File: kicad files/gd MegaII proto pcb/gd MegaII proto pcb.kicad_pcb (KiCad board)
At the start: 4 copper layers, 60 parts, among them J1 ABDIR, J10 Data, J11 PWR, J12 CLKS, J2 ABEN, J3 FLIP, J4 DBDIR, J5 DBEN, J6 VGC Extra 1, J7 Bald-Ext-1, J8 VGC Extra 2, J9 Address, U1 Apple_MEGA_II, U2 DRAM64KX4, U3 74HCT245, U4 DRAM64KX4, U5 74HCT245, U6 74HCT86, U7 DRAM64KX4, U8 74HCT245, U9 DRAM64KX4

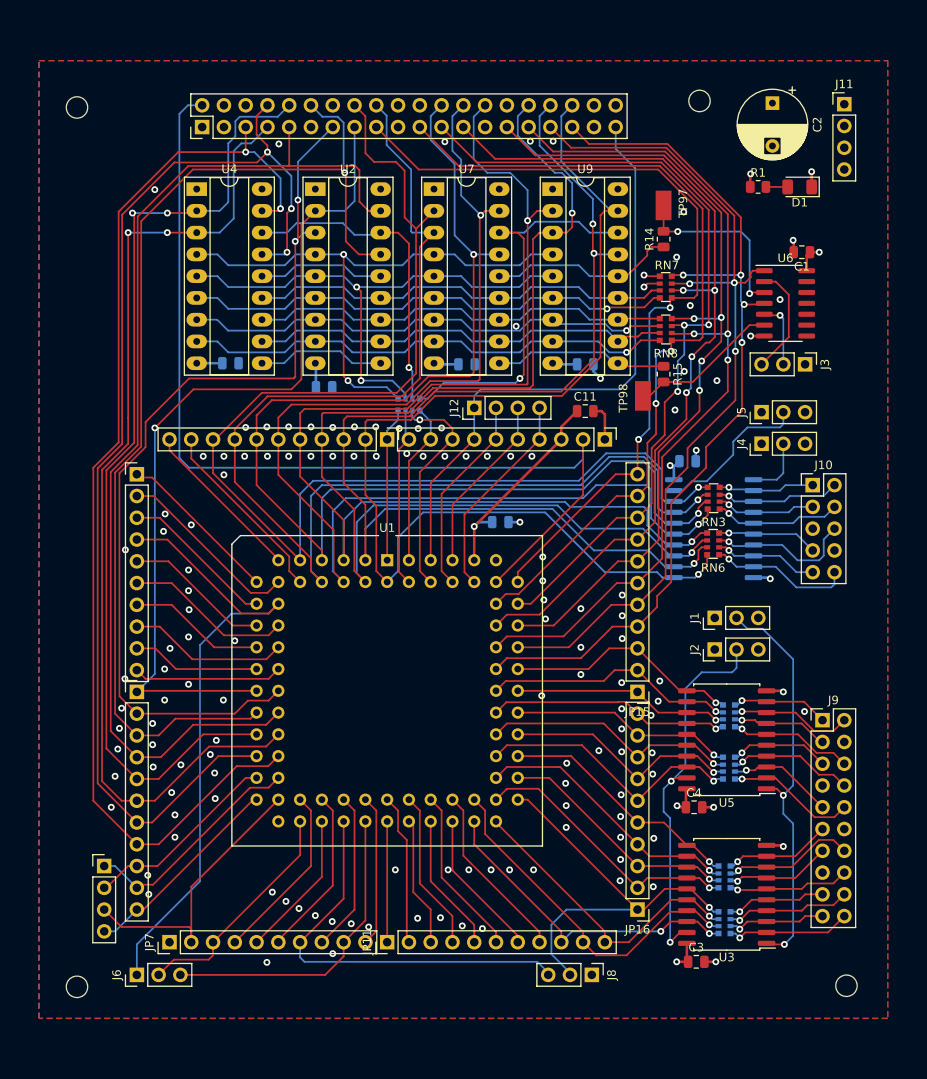
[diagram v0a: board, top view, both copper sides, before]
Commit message: all three boards final, prepping for gerbers
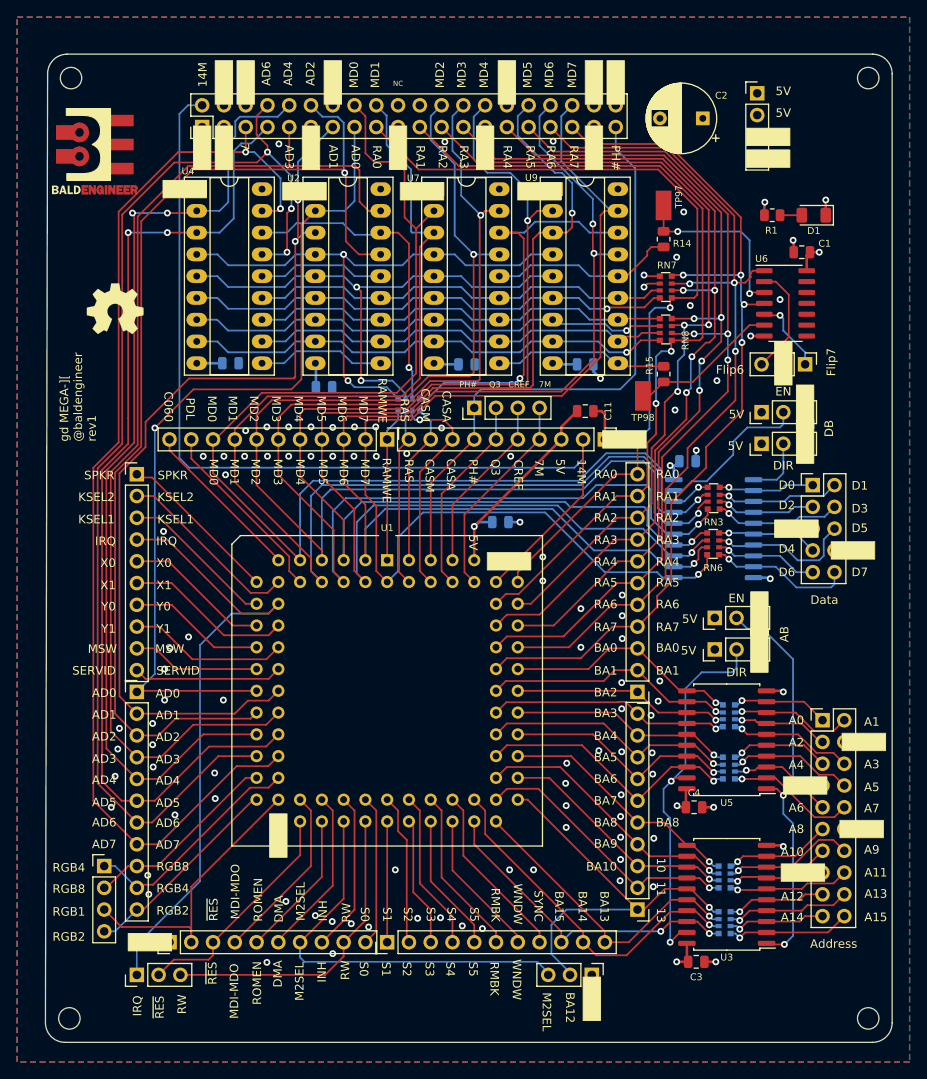
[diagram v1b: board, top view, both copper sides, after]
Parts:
- added REF**: OSHW-Symbol_6.7x6mm_SilkScreen, Symbol:OSHW-Symbol_6.7x6mm_SilkScreen, F.Cu at (97.8, 62.0)
- added REF**: KiCad-Logo_8mm_SilkScreen, Symbol:KiCad-Logo_8mm_SilkScreen, B.Cu at (129.8, 107.4)
- added svg2mod: G***, My Libraries:BE10v2, F.Cu at (90.4, 38.6)
- moved H2 19.9 mm to (185.7, 35.1)
- moved J11 10.2 mm to (172.7, 36.8)
- moved C2 8.32 mm to (166.4, 39.8), turned to 180 degrees
- moved H1 4.58 mm to (185.7, 144.8)
- moved H4 3.79 mm to (92.5, 144.8)
- moved D1 3.69 mm to (179.3, 51.1)
- moved R1 3.69 mm to (174.5, 51.1)
- moved H3 3.50 mm to (92.6, 35.1)
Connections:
- J3 pad 1: GND -> /FLIP7
- J3 pad 2: /FLIP7 -> GND
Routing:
- net /FLIP7: track 7.77 -> 8.82 mm
- net GND: vias 136 -> 99
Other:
- board outline added: 98.8 x 115.3 mm
- board text added: "1"
- board text added: "10"
- board text added: "11"
- board text added: "12"
- board text added: "13"
- board text added: "14M"
- board text added: "2"
- board text added: "24"
- board text added: "32"
- board text added: "39"
- board text added: "43"
- board text added: "44"
- board text added: "5"
- board text added: "53"
- board text added: "54"
- board text added: "5V"
- board text added: "64"
- board text added: "7"
- board text added: "7M"
- board text added: "A0"
- board text added: "A1"
- board text added: "A10"
- board text added: "A11"
- board text added: "A12"
- board text added: "A13"
- board text added: "A14"
- board text added: "A15"
- board text added: "A2"
- board text added: "A3"
- board text added: "A4"
- board text added: "A5"
- board text added: "A6"
- board text added: "A7"
- board text added: "A8"
- board text added: "A9"
- board text added: "AB"
- board text added: "AD0"
- board text added: "AD1"
- board text added: "AD2"
- board text added: "AD3"
- board text added: "AD4"
- board text added: "AD5"
- board text added: "AD6"
- board text added: "AD7"
- board text added: "Address"
- board text added: "BA0"
- board text added: "BA1"
- board text added: "BA10"
- board text added: "BA11"
- board text added: "BA12"
- board text added: "BA13"
- board text added: "BA14"
- board text added: "BA15"
- board text added: "BA2"
- board text added: "BA3"
- board text added: "BA4"
- board text added: "BA5"
- board text added: "BA6"
- board text added: "BA7"
- board text added: "BA8"
- board text added: "BA9"
- board text added: "C060"
- board text added: "CASA"
- board text added: "CASM"
- board text added: "CREF"
- board text added: "D0"
- board text added: "D1"
- board text added: "D2"
- board text added: "D3"
- board text added: "D4"
- board text added: "D5"
- board text added: "D6"
- board text added: "D7"
- board text added: "DB"
- board text added: "DIR"
- board text added: "DMA"
- board text added: "Data"
- board text added: "EN"
- board text added: "Flip6"
- board text added: "Flip7"
- board text added: "INH"
- board text added: "IRQ"
- board text added: "KSEL1"
- board text added: "KSEL2"
- board text added: "M2SEL"
- board text added: "MD0"
- board text added: "MD1"
- board text added: "MD2"
- board text added: "MD3"
- board text added: "MD4"
- board text added: "MD5"
- board text added: "MD6"
- board text added: "MD7"
- board text added: "MDI-MDO"
- board text added: "MSW"
- board text added: "NC"
- board text added: "PDL"
- board text added: "PH#"
- board text added: "Q3"
- board text added: "RA0"
- board text added: "RA1"
- board text added: "RA2"
- board text added: "RA3"
- board text added: "RA4"
- board text added: "RA5"
- board text added: "RA6"
- board text added: "RA7"
- board text added: "RAMWE"
- board text added: "RAS"
- board text added: "RGB1"
- board text added: "RGB2"
- board text added: "RGB4"
- board text added: "RGB8"
- board text added: "RMBK"
- board text added: "ROMEN"
- board text added: "RW"
- board text added: "S0"
- board text added: "S1"
- board text added: "S2"
- board text added: "S3"
- board text added: "S4"
- board text added: "S5"
- board text added: "SERVID"
- board text added: "SPKR"
- board text added: "SYNC"
- board text added: "This board (and this project) would not happen without the help of rjhelms. Thank you!"
- board text added: "U2"
- board text added: "U4"
- board text added: "U7"
- board text added: "U9"
- board text added: "WNDW"
- board text added: "X0"
- board text added: "X1"
- board text added: "Y0"
- board text added: "Y1"
- board text added: "gd MEGA-][ @baldengineer rev1"
- board text added: "~RES"
